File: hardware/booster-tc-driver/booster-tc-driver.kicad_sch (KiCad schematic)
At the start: 133 parts, among them IC1 AD5160BRJZ5-RL7, IC2 AD5160BRJZ5-RL7, IC3 BD50FD0WHFP-TR, IC4 CAT4109V-GT2, J1 62201021121, J10 3-647166-2, J2 EHT-105-01-S-D, J3 3-647166-2, J6 22-23-2021, J7 3-647166-2, J8 B4B-PH-SM4-TB, Q1 T2N7002AK, Q2 NTR5198NLT1G, SW1 SW_SPDT, U1 STM32G474CBTx, U10 LT1963AxST-3.3, U11 AP1501A-12K5G-13, U2 AOZ1284PI, U3 CSTNE8M00G550000R0, U4 IF-D95T << must be T, U5 IF-E96E, U6 IF-D95T << must be T, U7 AOZ1284PI

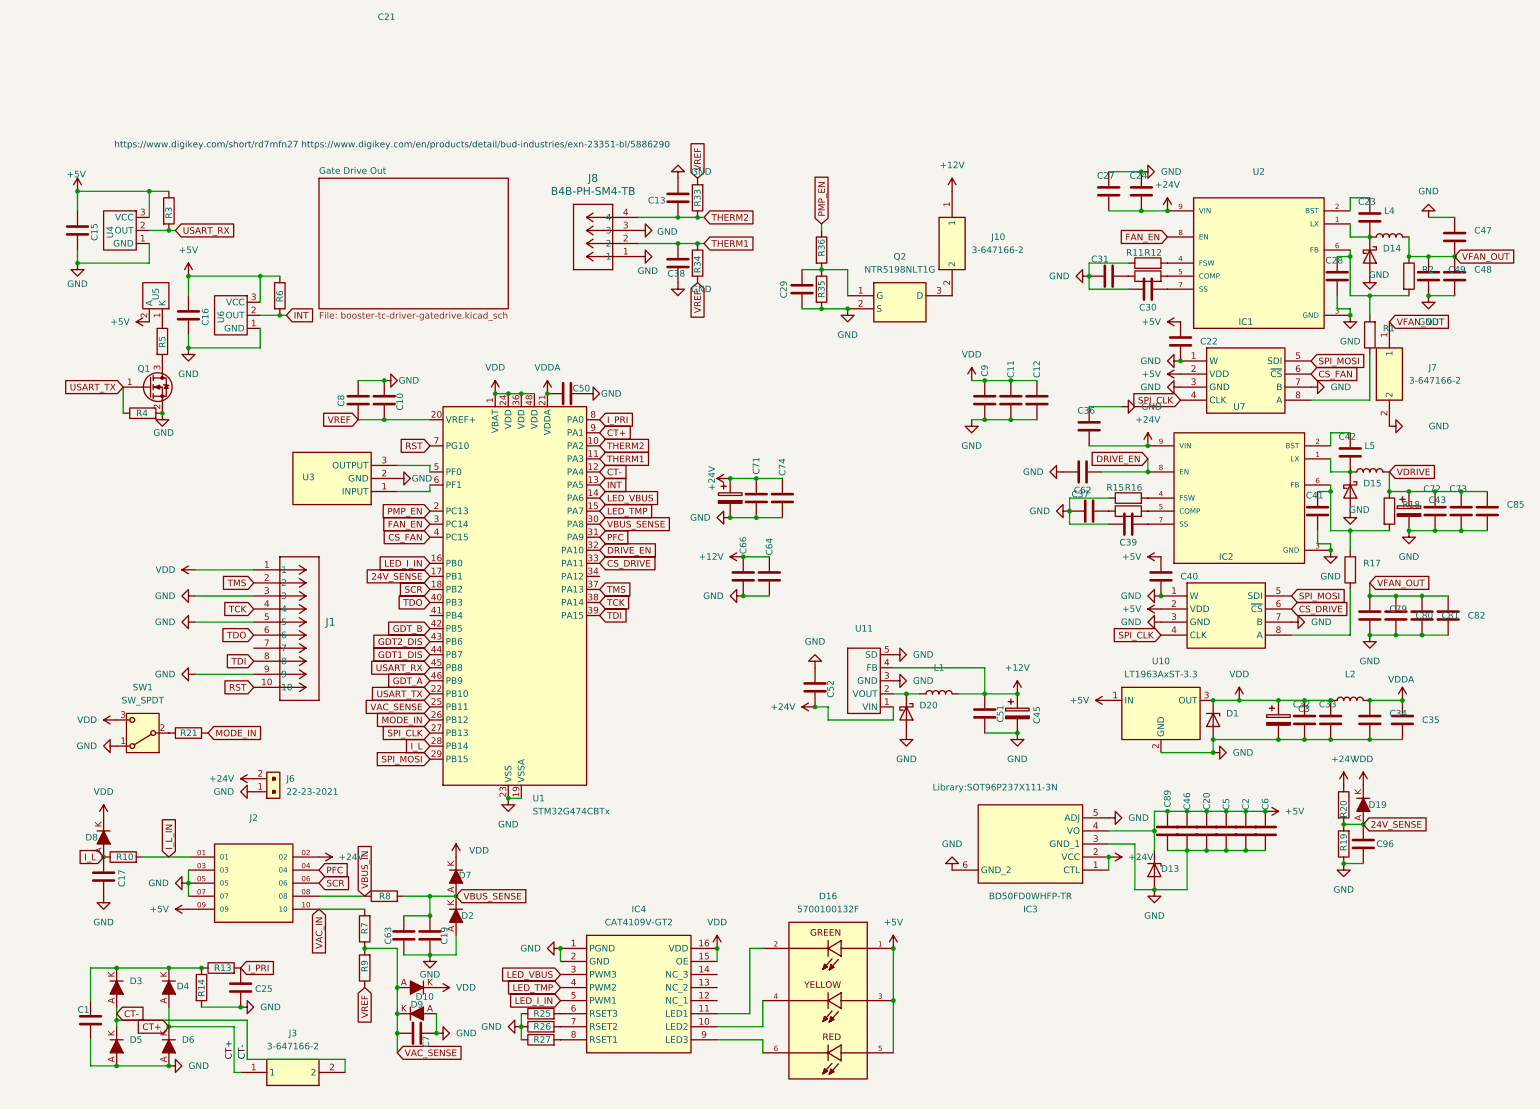
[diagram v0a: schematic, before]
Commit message: ftdi board + random stuff
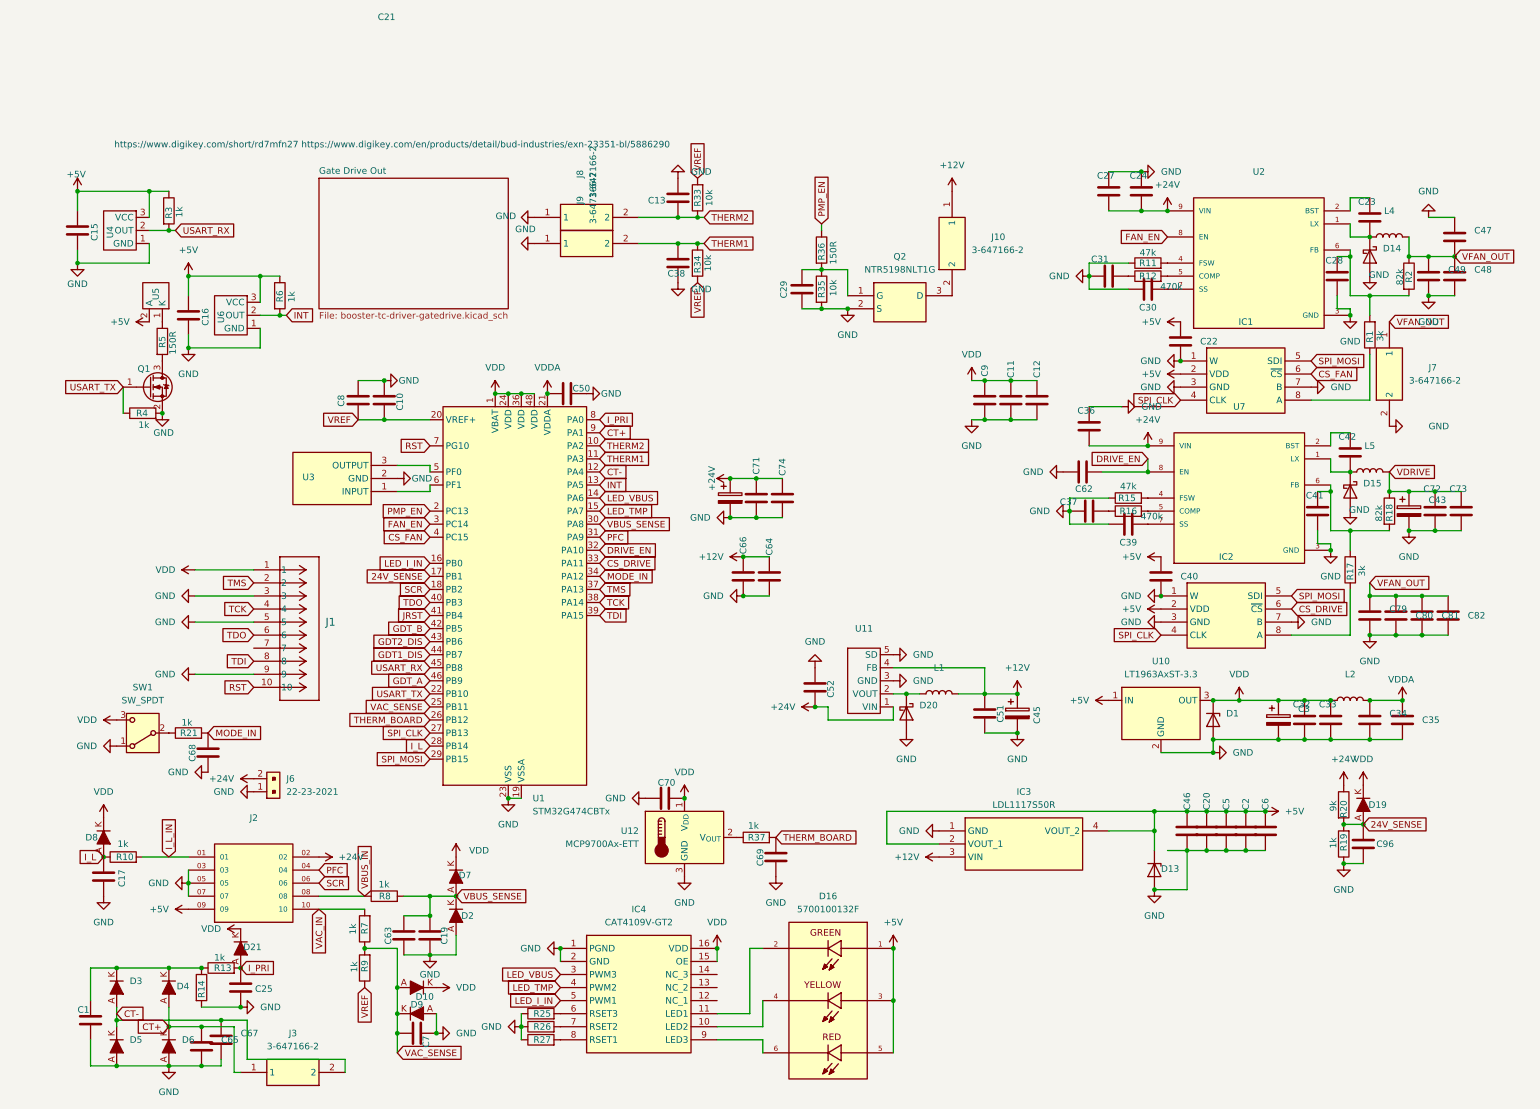
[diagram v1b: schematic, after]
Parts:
- removed C85, C89: 2u2 C3225X7R1H225K250AB, Capacitor_SMD:C_1210_3225Metric_Pad1.33x2.70mm_HandSolder, symbol Device:C
- removed IC3: BD50FD0WHFP-TR, Library:BD50FD0WHFPTR, symbol New_Library:BD50FD0WHFP-TR
- removed J8: B4B-PH-SM4-TB, Library:CONN_B4B-PH-SM4-TB_JST, symbol New_Library:B4B-PH-SM4-TB
- added C65, C67: 150p VJ0603A151JXAAC, Capacitor_SMD:C_0603_1608Metric_Pad1.08x0.95mm_HandSolder, symbol Device:C
- added C68, C69: 10n VJ0603Y103KXJAC31X, Capacitor_SMD:C_0603_1608Metric_Pad1.08x0.95mm_HandSolder, symbol Device:C
- added C70: .1uf 885012208087, Capacitor_SMD:C_1206_3216Metric_Pad1.33x1.80mm_HandSolder, symbol Device:C
- added D21: MBR0530, digikey-footprints:SOD-123, symbol dk_Diodes-Rectifiers-Single:1N5819HW-7-F
- added IC3: LDL1117S50R, SOT230P700X180-4N, symbol New_Library:LDL1117S50R
- added J8, J9: 3-647166-2, Library:36471662, symbol New_Library:3-647166-2
- added R37: 1k, Resistor_SMD:R_0805_2012Metric_Pad1.20x1.40mm_HandSolder, symbol Device:R
- added U12: MCP9700Ax-ETT, Package_TO_SOT_SMD:SOT-23, symbol Sensor_Temperature:MCP9700Ax-ETT
- R1, R17: value 3k CRCW08053K00FKTA -> 3k
- R10, R13, R19, R21, R3, R4, R6, R7, R8, R9: value 1k MCU0805MD1051BP500 -> 1k
- R11, R15: value 47k CRCW080547K0FKEA -> 47k
- R12, R16: value 470k CRCW0805470KFKTA -> 470k
- R14: value 5R1 ERJ-B1BF5R1U -> 2R2 35222R2JT; footprint Resistor_SMD:R_1020_2550Metric_Pad1.33x5.20mm_HandSolder -> Resistor_SMD:R_2512_6332Metric_Pad1.40x3.35mm_HandSolder
- R18, R2: value 82k CRCW080582K0FKEA -> 82k
- R20: value 9k CRCW08059K10FKEAHP -> 9k
- R33, R34, R35: value 10k CRCW080510K0DHEAP -> 10k
- R36, R5: value 150R KTR18EZPJ151 -> 150R; footprint Resistor_SMD:R_1206_3216Metric_Pad1.30x1.75mm_HandSolder -> Resistor_SMD:R_0805_2012Metric_Pad1.20x1.40mm_HandSolder
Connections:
- net +12V: now also IC3.3 (VIN)
- net +5V: now also IC3.2 (VOUT_1), IC3.4 (VOUT_2)
- net CT+: now also C65.1
- net CT-: now also C67.1
- net GND: now also C65.2, C67.2, C68.2, C69.2, C70.1, IC3.1 (GND), J8.1, J9.1, U12.3 (GND)
- net I_PRI: now also D21.A
- net MODE_IN: now also U1.34 (PA12), C68.1; no longer U1.26 (PB12)
- net THERM1: now also J9.2
- net THERM2: now also J8.2
- net VDD: now also C70.2, D21.K, U12.1 (V_{DD})
- net JRST: now reaches U1.41 (PB4)
- new net: R37.1, U12.2 (V_{OUT})
- new net THERM_BOARD: C69.1, R37.2, U1.26 (PB12)
